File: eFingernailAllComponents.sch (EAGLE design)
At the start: 5 parts, among them IC1 74HC595D, U2 52892-1695, U3 Tiny85-20-SMT

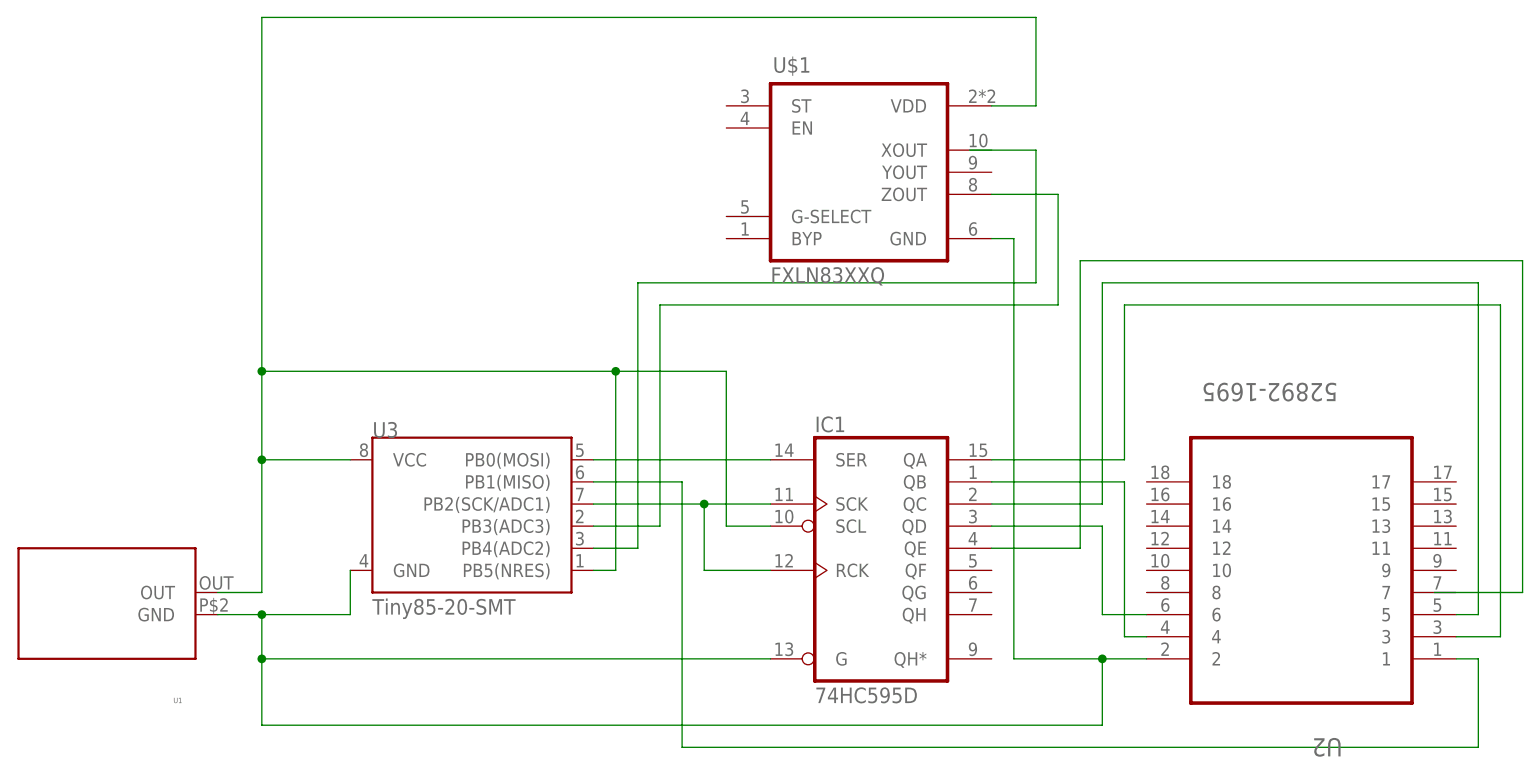
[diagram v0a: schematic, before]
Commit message: latest board
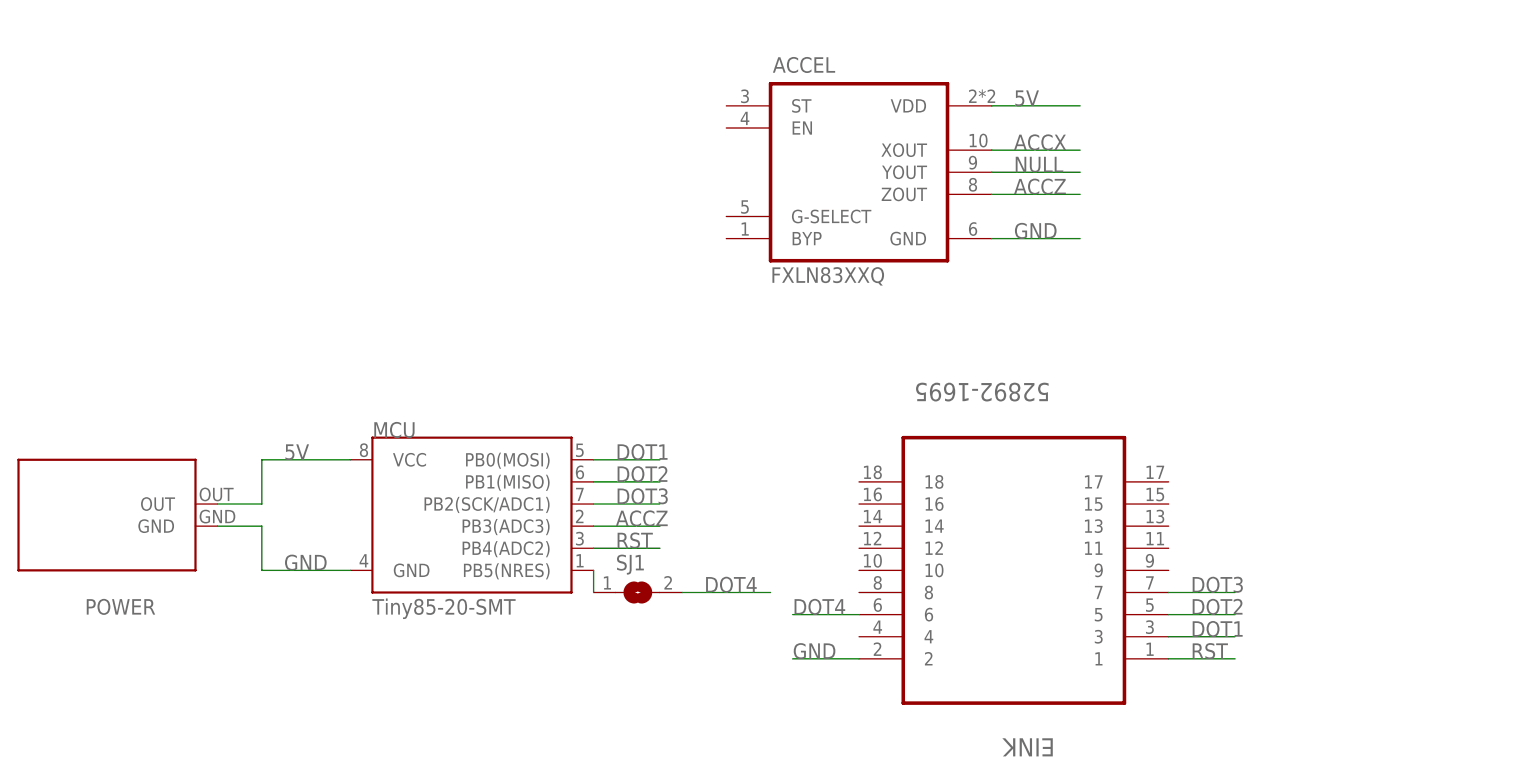
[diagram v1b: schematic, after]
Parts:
- removed IC1: 74HC595D, 74xx:74HC595D
- removed U1: (no value), GeekAmmo:P9027LP-R
- removed U2: 52892-1695, Molex_By_element14_Batch_1:52892-1695
- added EINK: 52892-1695, Molex_By_element14_Batch_1:52892-1695
- added POWER: (no value), PowerReceiver:P9027LP-R
- added SJ1: (no value), microbuilder:SOLDERJUMPER
- renumbered U$1 to ACCEL, U3 to MCU
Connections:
- net N$11 renamed ACCZ
- removed net N$10: IC1A.QE
- removed net N$12: MCU.PB4(ADC2)
- removed net N$2: ACCEL.GND, IC1A.G, MCU.GND, U1.GND, U2.2
- removed net N$3: IC1A.RCK, IC1A.SCK, MCU.PB2(SCK/ADC1)
- removed net N$4: IC1A.SER, MCU.PB0(MOSI)
- removed net N$5: IC1A.QA, U2.3
- removed net N$6: MCU.PB1(MISO), U2.1
- removed net N$7: IC1A.QB, U2.4
- removed net N$8: IC1A.QC, U2.5
- removed net N$9: IC1A.QD, U2.6
- new net 5V: ACCEL.VDD, MCU.VCC, POWER.OUT
- new net ACCX: ACCEL.XOUT
- new net DOT1: EINK.3, MCU.PB0(MOSI)
- new net DOT2: EINK.5, MCU.PB1(MISO)
- new net DOT3: EINK.7, MCU.PB2(SCK/ADC1)
- new net DOT4: EINK.6, SJ1.2
- new net GND: ACCEL.GND, EINK.2, MCU.GND, POWER.GND
- new net NULL: ACCEL.YOUT
- new net RST: EINK.1, MCU.PB4(ADC2)
- net N$1: now also SJ1.1; no longer ACCEL.VDD, IC1A.SCL, MCU.VCC, U1.OUT
